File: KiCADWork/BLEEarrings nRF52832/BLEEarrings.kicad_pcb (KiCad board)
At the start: 2 copper layers, 25.5 x 37.8 mm, 48 parts, among them J1 Screw_Terminal_01x01, J2 Screw_Terminal_01x02, J3 USB_C_Receptacle, SW1 TK-6580B-1, SW2 SW_DIP_x01, U1 MCP73831T-2ACI/OT, U2 XB6096I2SV, U3 NRF52833-QDAA-R7, Y1 XL7EL89CKI-111YLC-32M, Y2 X161032768KLD2SI

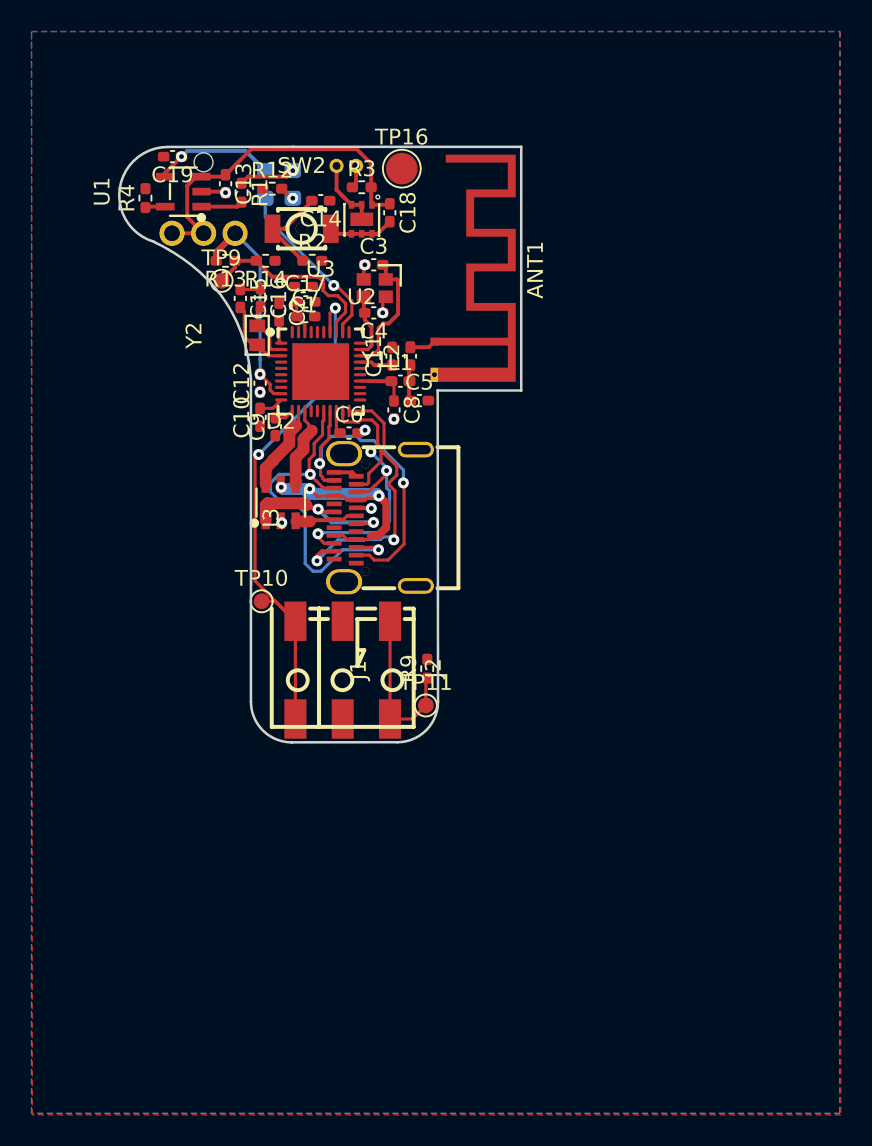
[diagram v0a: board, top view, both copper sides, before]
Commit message: Ignoring Backups
More Dock progress
All local backups removed
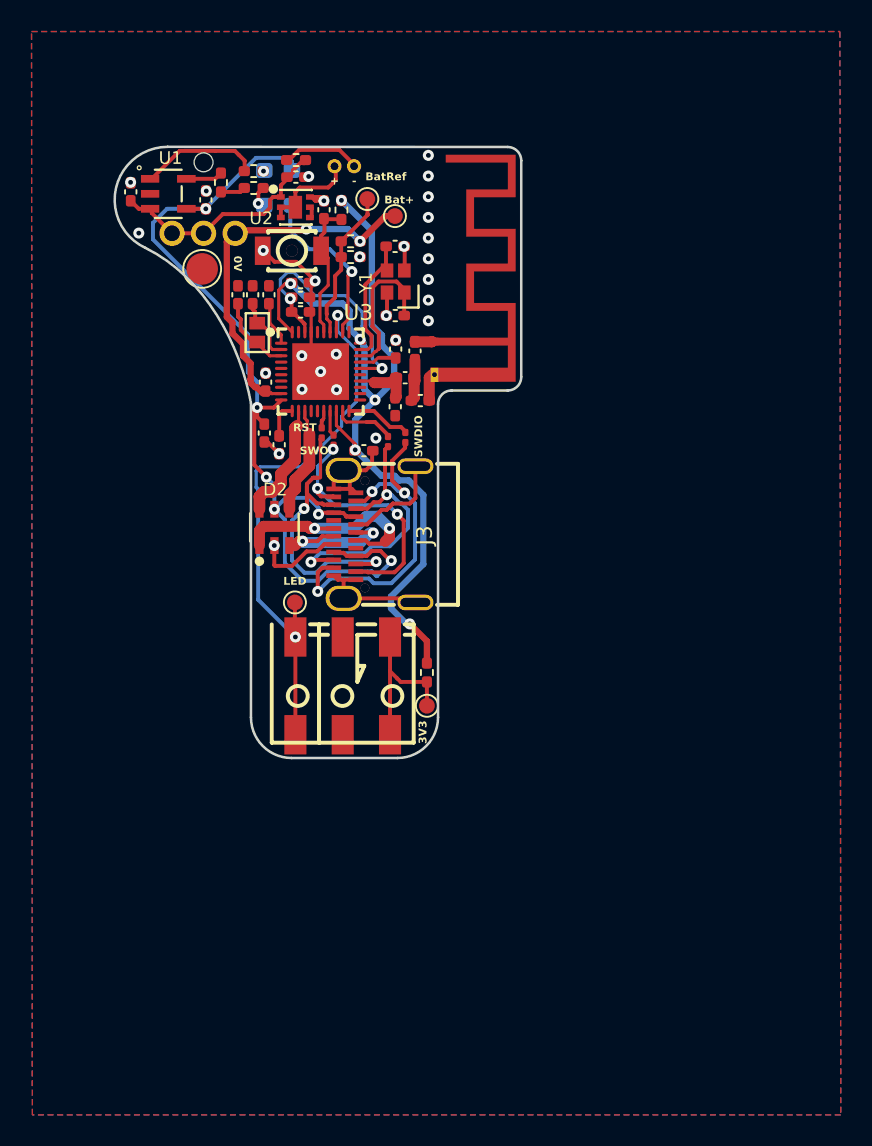
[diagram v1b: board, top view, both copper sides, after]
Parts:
- added G***: LOGO, CustomPads:DK6, B.Cu at (145.8, 58.4)
- added R5: NF, Resistor_SMD:R_0201_0603Metric, F.Cu at (142.8, 60.2)
- added R6: NF, Resistor_SMD:R_0201_0603Metric, F.Cu at (143.5, 60.6)
- added R7: NF, Resistor_SMD:R_0201_0603Metric, F.Cu at (148.1, 60.5)
- added R8: NF, Resistor_SMD:R_0201_0603Metric, F.Cu at (146.9, 60.7)
- added TP1: TestPoint, TestPoint:TestPoint_Pad_D1.0mm, F.Cu at (147.4, 46.4)
- moved TP16 14.2 mm to (135.2, 49.8)
- moved TP9 10.6 mm to (145.6, 45.4)
- moved R13 8.03 mm to (144.6, 48.0), turned to 0 degrees
- moved C18 6.37 mm to (141.1, 44.0), turned to 0 degrees
- moved C13 6.03 mm to (130.6, 44.9), turned to 90 degrees
- moved R14 5.40 mm to (144.6, 49.0)
- moved R4 4.89 mm to (136.4, 44.3), turned to -90 degrees
- moved R3 4.51 mm to (141.1, 42.9)
- moved C4 4.43 mm to (147.4, 48.4)
- moved U2 4.28 mm to (141.1, 45.9), turned to -90 degrees
- moved R2 3.71 mm to (144.0, 46.1), turned to 90 degrees
- moved C3 3.50 mm to (147.4, 52.8)
- moved C19 3.46 mm to (135.4, 45.4), turned to 90 degrees
- moved TP10 2.11 mm to (141.1, 70.9)
- moved D2 1.62 mm to (139.8, 66.2)
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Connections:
- J3 pad A10: nRESET -> /DSP/nReset
- J3 pad A11: SWO -> SWO_L
- J3 pad A2: SWDIO -> SWDIO_L
- J3 pad A3: SWDCLK -> SWDCLK_L
- J3 pad B10: nRESET -> /DSP/nReset
- J3 pad B11: SWO -> SWO_L
- J3 pad B2: SWDIO -> SWDIO_L
- J3 pad B3: SWDCLK -> SWDCLK_L
- U3 pad 16: nRESET -> Net-(U3-P0.18_nRESET)
- U3 pad 17: SWO -> Net-(U3-P0.20)
- U3 pad 19: SWDCLK -> Net-(U3-SWDIO)
- U3 pad 20: SWDIO -> Net-(U3-SWDCLK)
- U3 pad 33: BatRef -> NEO_LED
- U3 pad 34: NEO_LED -> BatRef
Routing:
- net +3V3: track 1.88 -> 54.1 mm, vias 0 -> 6
- net GND: track 12.9 -> 48.4 mm, vias 8 -> 29
- net /DSP/VBUS: track 27.0 -> 59.1 mm, vias 4 -> 6
- net nRESET: track 22.5 -> 0.00 mm, vias 2 -> 0
- net SWDIO_L: track 0.00 -> 22.1 mm, vias 0 -> 3
- net SWO: track 22.0 -> 0.00 mm, vias 2 -> 0
- net SWDIO: track 21.1 -> 0.00 mm, vias 2 -> 0
- net SWDCLK: track 19.0 -> 0.00 mm, vias 3 -> 0
- net /DSP/nReset: track 0.00 -> 18.7 mm, vias 0 -> 2
- net SWDCLK_L: track 0.00 -> 16.9 mm, vias 0 -> 2
- net SWO_L: track 0.00 -> 16.9 mm, vias 0 -> 3
- net DEC6: track 2.18 -> 16.2 mm, vias 0 -> 2
- net +BATT: track 13.9 -> 23.8 mm, vias 1 -> 2
- net /Power/VBAT: track 22.2 -> 14.9 mm
- net Net-(U1-STAT): track 2.66 -> 7.54 mm
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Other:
- board size 25.5 x 37.8 mm -> 25.8 x 38.8 mm
- board text added: "+"
- board text added: "-"
- board text added: "0V"
- board text added: "3V3"
- board text added: "Bat+"
- board text added: "BatRef"
- board text added: "DK"
- board text added: "LED"
- board text added: "RST"
- board text added: "SWDIO"
- board text added: "SWO"
- board text added: "V1"
- board text added: "o o ← Brainwashing Rays → o"
